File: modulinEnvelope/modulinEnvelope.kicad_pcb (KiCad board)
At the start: 2 copper layers, 50.8 x 177.8 mm, 52 parts, among them J1 Screw_Terminal_01x06, Q1 BC548, Q2 BC548, Q3 BC548, Q4 BC548, Q5 BC548, Q6 BC548, Q7 2N7000, U1 TL074, U2 NA555P

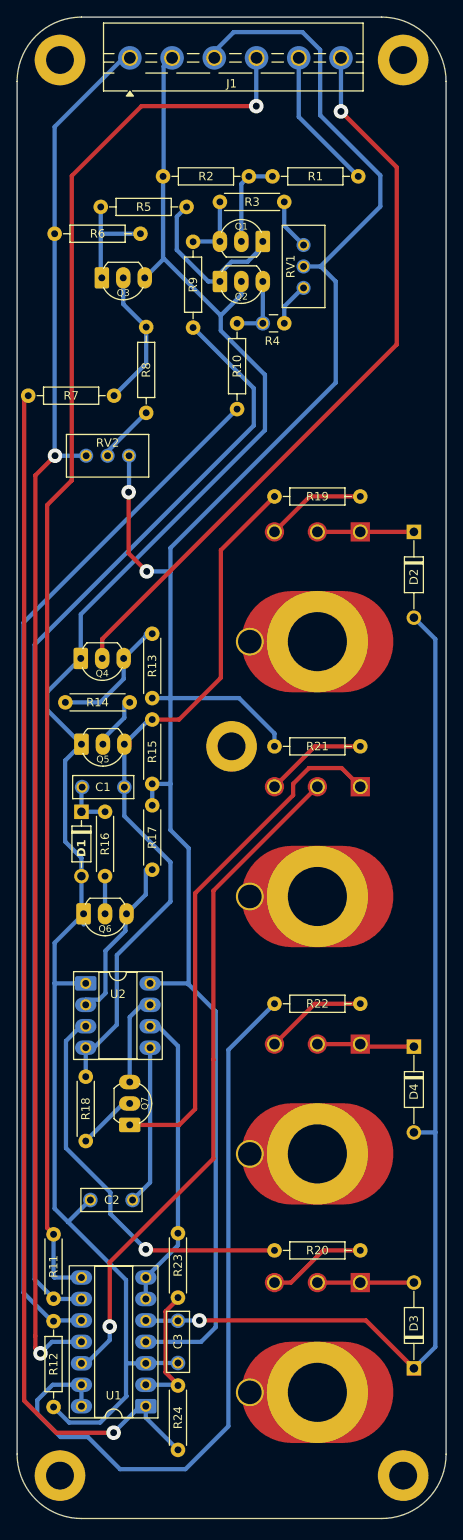
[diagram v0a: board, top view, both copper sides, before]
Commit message: Add STEP files
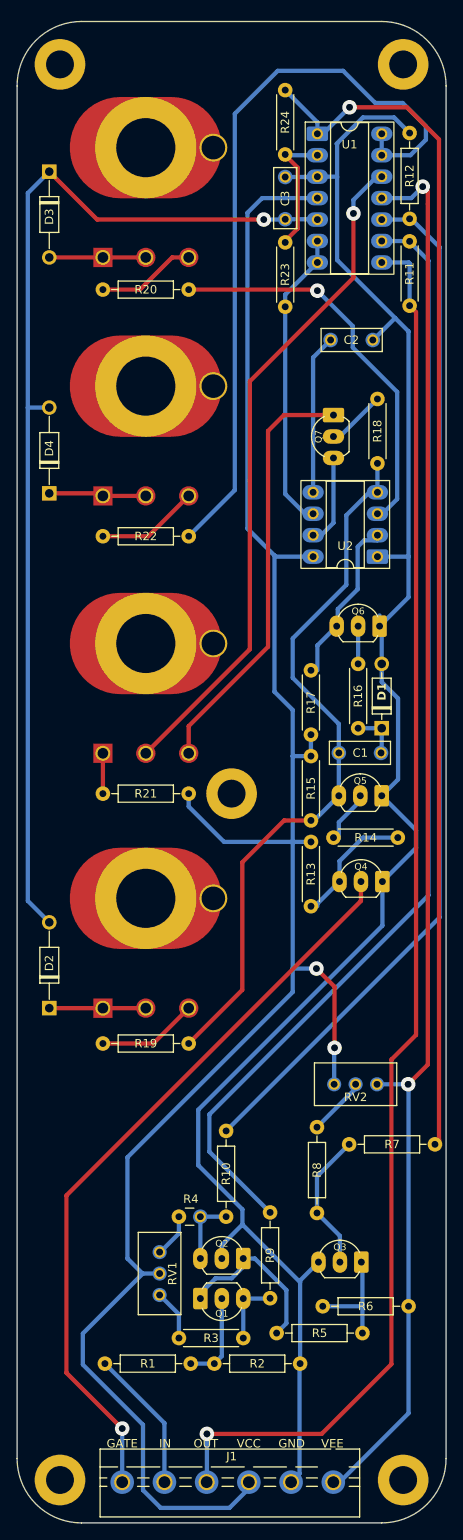
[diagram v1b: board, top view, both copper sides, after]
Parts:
- moved REF** 173.0 mm to (71.1, 188.5), turned to 90 degrees
- moved REF** 173.0 mm to (30.5, 188.5), turned to 90 degrees
- moved REF** 172.0 mm to (30.5, 20.8), turned to 90 degrees
- moved REF** 172.0 mm to (71.1, 20.8), turned to 90 degrees
- moved J1 170.4 mm to (62.8, 188.7), turned to 180 degrees
- moved R24 161.5 mm to (57.1, 23.9), turned to -90 degrees
- moved U1 152.0 mm to (61.0, 29.1), turned to 0 degrees
- moved RV4 148.8 mm to (40.6, 30.7), turned to 180 degrees
- moved D3 148.2 mm to (29.2, 33.5), turned to -90 degrees
- moved R2 141.5 mm to (58.9, 174.7), turned to 180 degrees
- moved C3 141.0 mm to (57.1, 34.2), turned to -90 degrees
- moved R1 140.9 mm to (46.0, 174.7), turned to 180 degrees
- moved R12 137.2 mm to (71.9, 39.1), turned to 90 degrees
- moved R5 136.9 mm to (66.3, 171.1), turned to 180 degrees
- moved R3 134.6 mm to (52.2, 171.7), turned to 180 degrees
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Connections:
- RV5 pad 1: Net-(R21-Pad2) -> Net-(Q7-D)
- RV5 pad 3: Net-(Q7-D) -> Net-(R21-Pad2)
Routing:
- net Net-(Q7-D): track 61.5 -> 50.6 mm
- net Net-(R21-Pad2): track 12.1 -> 4.78 mm
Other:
- board text added: "GATE"
- board text added: "GND"
- board text added: "IN"
- board text added: "OUT"
- board text added: "VCC"
- board text added: "VEE"
